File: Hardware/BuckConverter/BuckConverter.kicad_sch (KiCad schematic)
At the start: 10 parts, among them J2 Screw_Terminal_01x02, Q1 DMT6012LSS, Q2 DMT6012LSS, U1 LTC4444-5

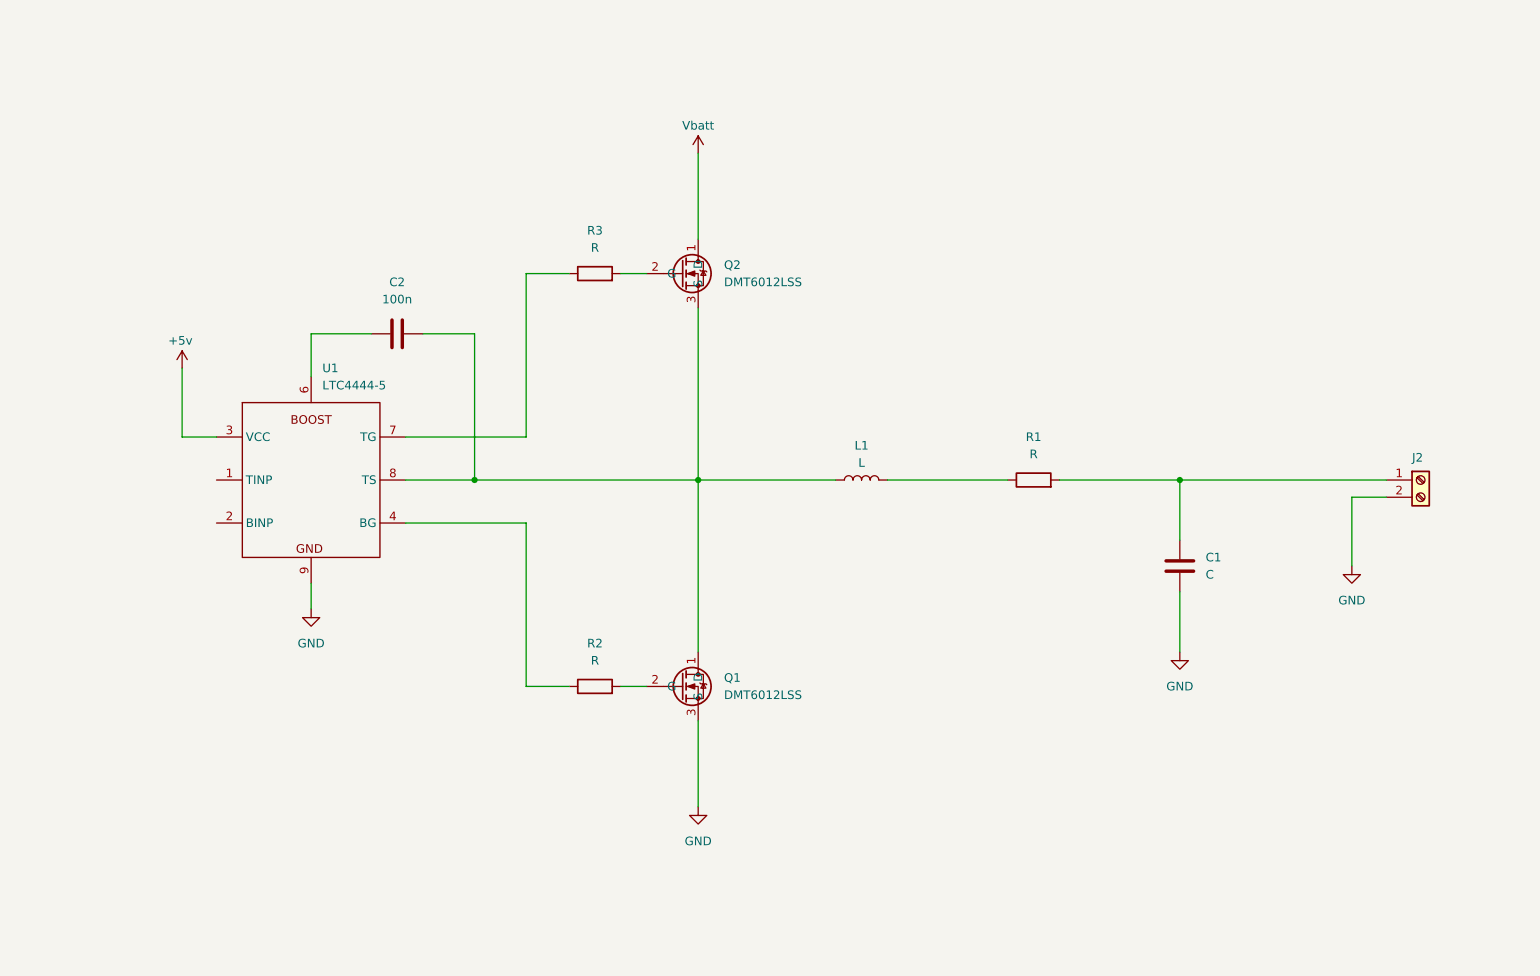
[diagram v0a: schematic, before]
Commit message: buck converter V1
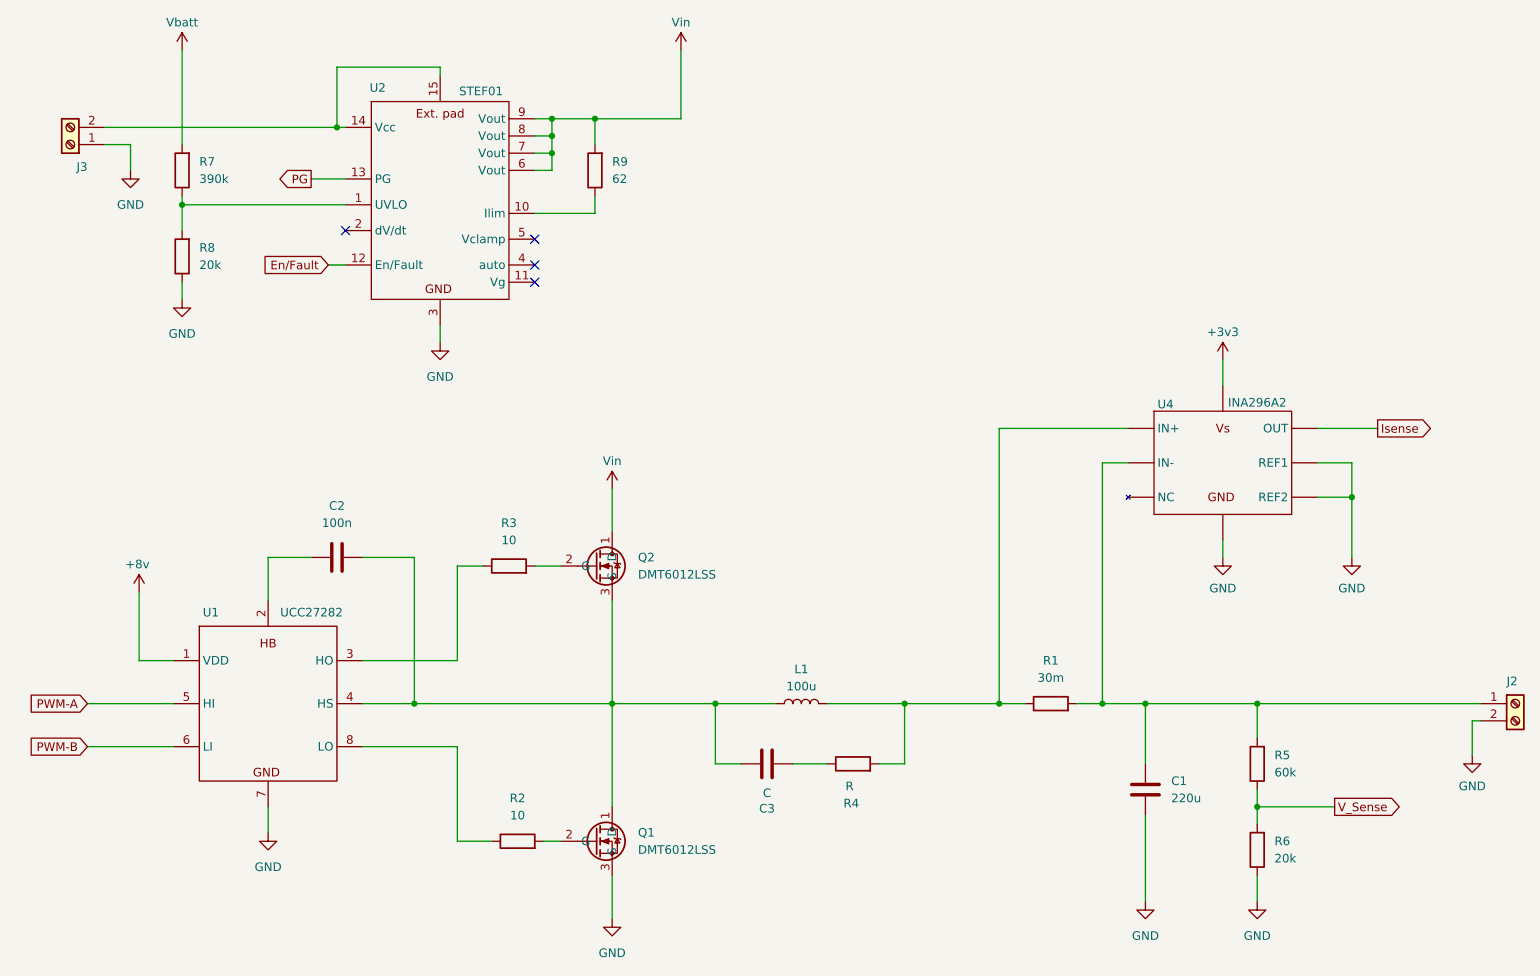
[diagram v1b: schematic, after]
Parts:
- removed U1: LTC4444-5, symbol KicadLib:LTC4444-5
- added C3: C, symbol Device:C
- added J3: Screw_Terminal_01x02, symbol Connector:Screw_Terminal_01x02
- added R4: R, symbol Device:R
- added R5: 60k, symbol Device:R
- added R6, R8: 20k, symbol Device:R
- added R7: 390k, symbol Device:R
- added R9: 62, symbol Device:R
- added U1: UCC27282, kicadLibFp:SOIC-8, symbol KicadLib:UCC27282
- added U2: STEF01, symbol KicadLib:STEF01
- added U4: INA296A2, symbol KicadLib:INA296A2
- C1: value C -> 220u
- L1: value L -> 100u
- R1: value R -> 30m
- R2, R3: value R -> 10
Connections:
- net GND: now also J3.1 (Pin_1), R6.1, R8.1, U1.7, U2.3, U4. (REF2)
- net Vbatt: now also R7.2; no longer Q2.1 (D)
- net at C2.1: now also U1.2
- net at C2.2, L1.1, Q1.1 (D)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: now also C3.2, U1.4 (HS)
- net at L1.2, R1.1: now also R4.2, U4. (REF2)
- net at R2.1: now also U1.8 (LO)
- net at R3.1: now also U1.3 (HO)
- net at C1.1, J2.1 (Pin_1), R1.2: now also R5.2, U4. (REF2)
- new net: R7.1, R8.2, U2.1 (UVLO)
- new net: R9.1, U2.10 (Ilim)
- new net: C3.1, R4.1
- new net: J3.2 (Pin_2), U2.14 (Vcc), U2.15
- new net +3v3: U4. (REF2)
- new net +8v: U1.1 (VDD)
- new net En/Fault: U2.12 (En/Fault)
- new net Isense: U4. (REF2)
- new net PG: U2.13 (PG)
- new net PWM-A: U1.5 (HI)
- new net PWM-B: U1.6 (LI)
- new net V_Sense: R5.1, R6.2
- new net Vin: Q2.1 (D), R9.2, U2.6 (Vout), U2.7 (Vout), U2.8 (Vout), U2.9 (Vout)
- no-connect marks 0 -> 4
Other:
- moved on the sheet: C1, C2, J2, L1, Q1, Q2, R1, R2, R3
